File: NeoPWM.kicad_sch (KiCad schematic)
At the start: 0 parts

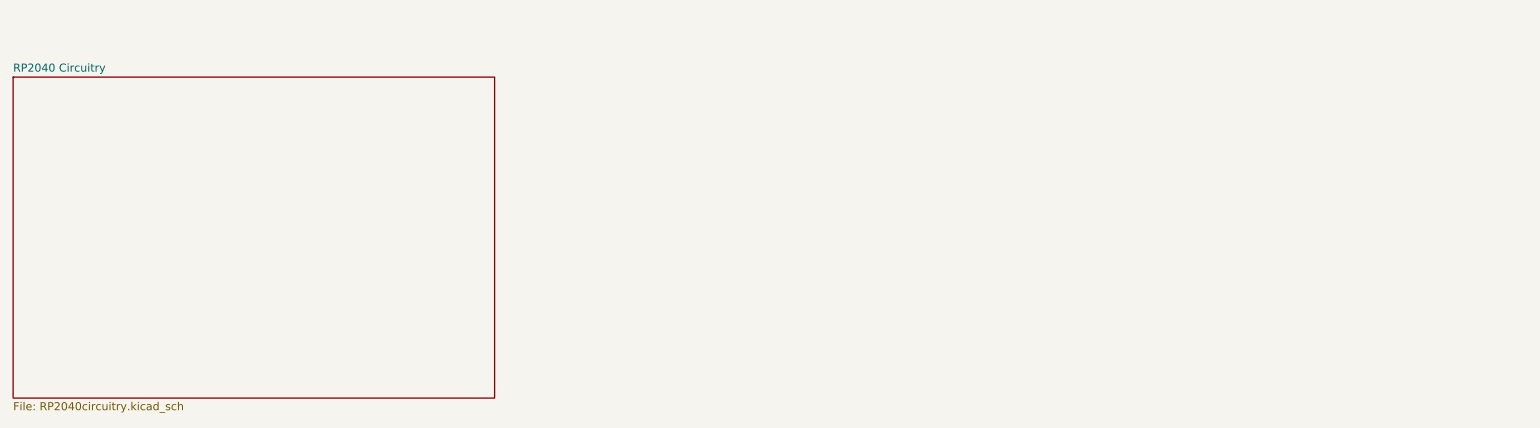
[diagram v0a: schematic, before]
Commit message: Power + Optocoupler
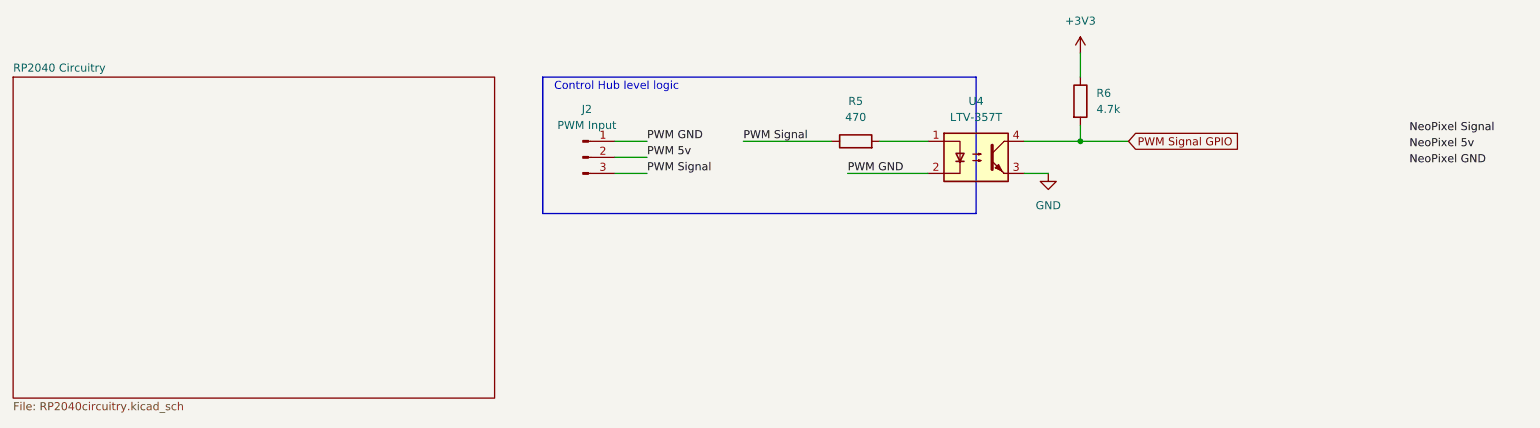
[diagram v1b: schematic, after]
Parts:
- added J2: PWM Input, Connector:FanPinHeader_1x03_P2.54mm_Vertical, symbol Connector:Conn_01x03_Pin
- added R5: 470, symbol Device:R
- added R6: 4.7k, symbol Device:R
- added U4: LTV-357T, Package_DIP:DIP-4_W7.62mm, symbol Isolator:LTV-357T
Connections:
- new net: R5.2, U4.1
- new net +3V3: R6.1
- new net GND: U4.3
- new net PWM 5v: J2.2 (Pin_2)
- new net PWM GND: J2.1 (Pin_1), U4.2
- new net PWM Signal: J2.3 (Pin_3), R5.1
- new net PWM Signal GPIO: R6.2, U4.4
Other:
- note added: "Control Hub level logic"
